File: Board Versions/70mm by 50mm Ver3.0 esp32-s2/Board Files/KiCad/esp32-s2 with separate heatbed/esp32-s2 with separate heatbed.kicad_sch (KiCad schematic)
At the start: 24 parts, among them IC1 ESP32-S2FN4R2, J1 PJ-037B, J2 USB4520-03-0-A, U1 LD1117S33TR_SOT223, U2 MAX31855KASA, Y1 ECS-400-15-33B-CTN-TR

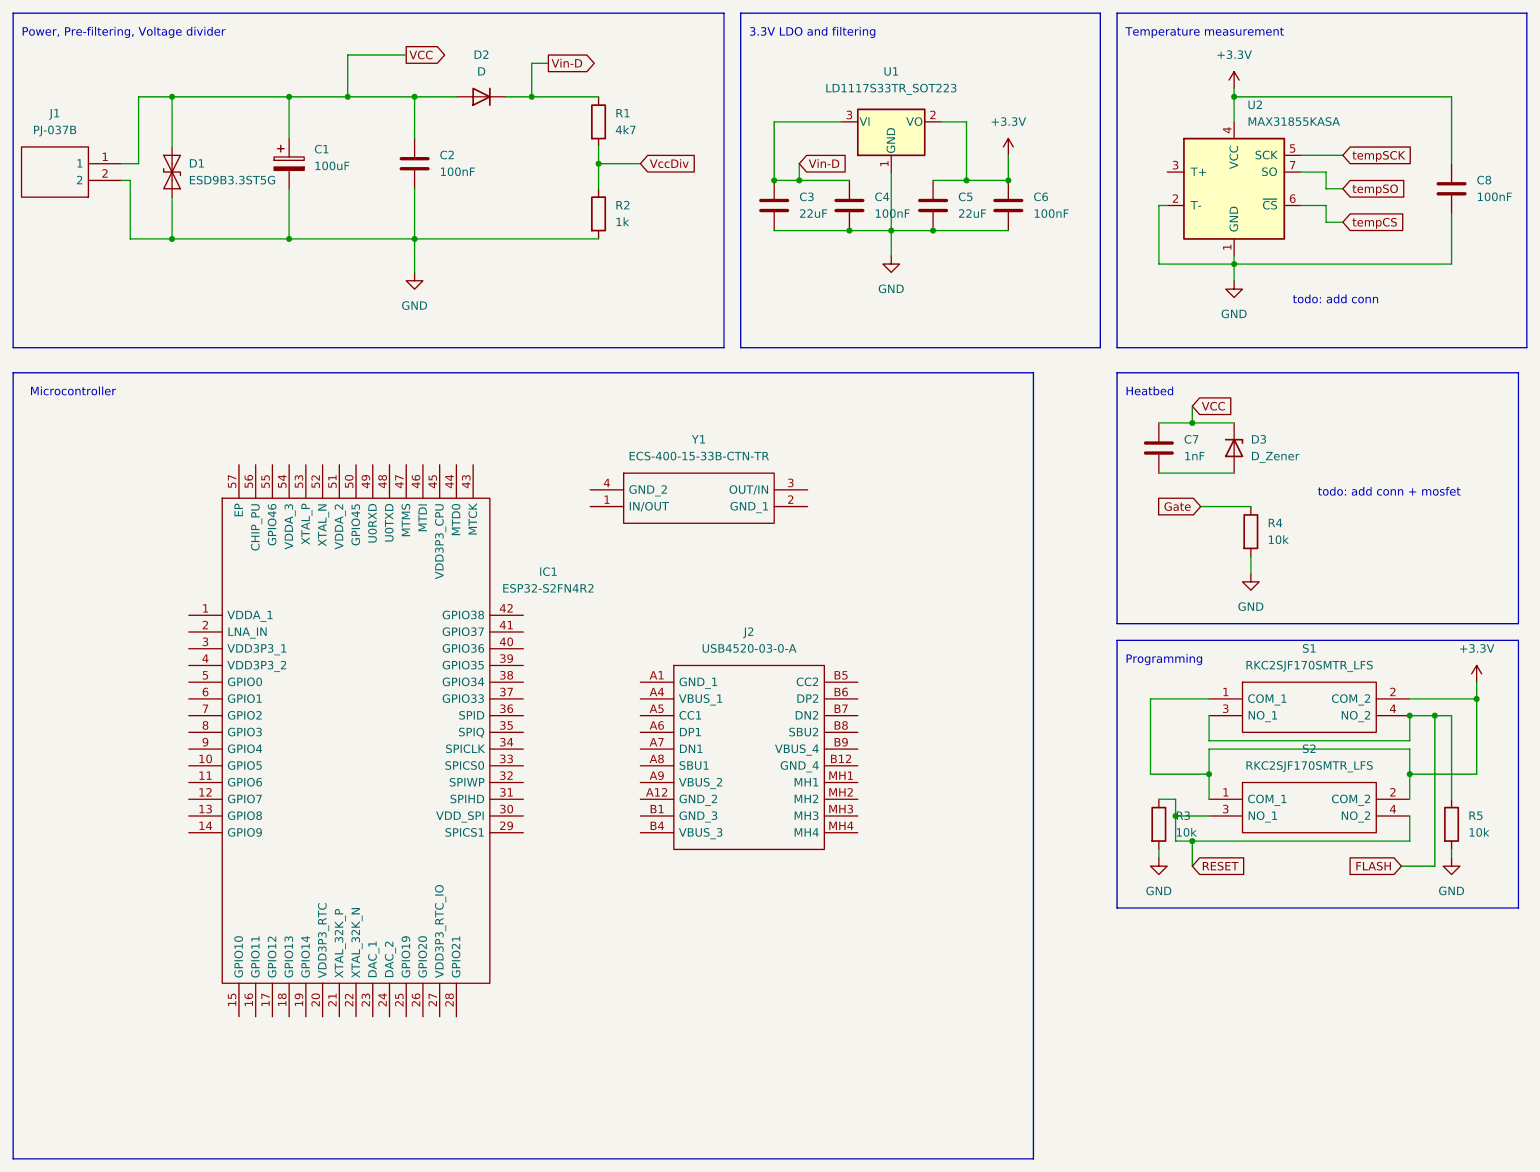
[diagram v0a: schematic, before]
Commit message: Microcontrolling schematics, not complete
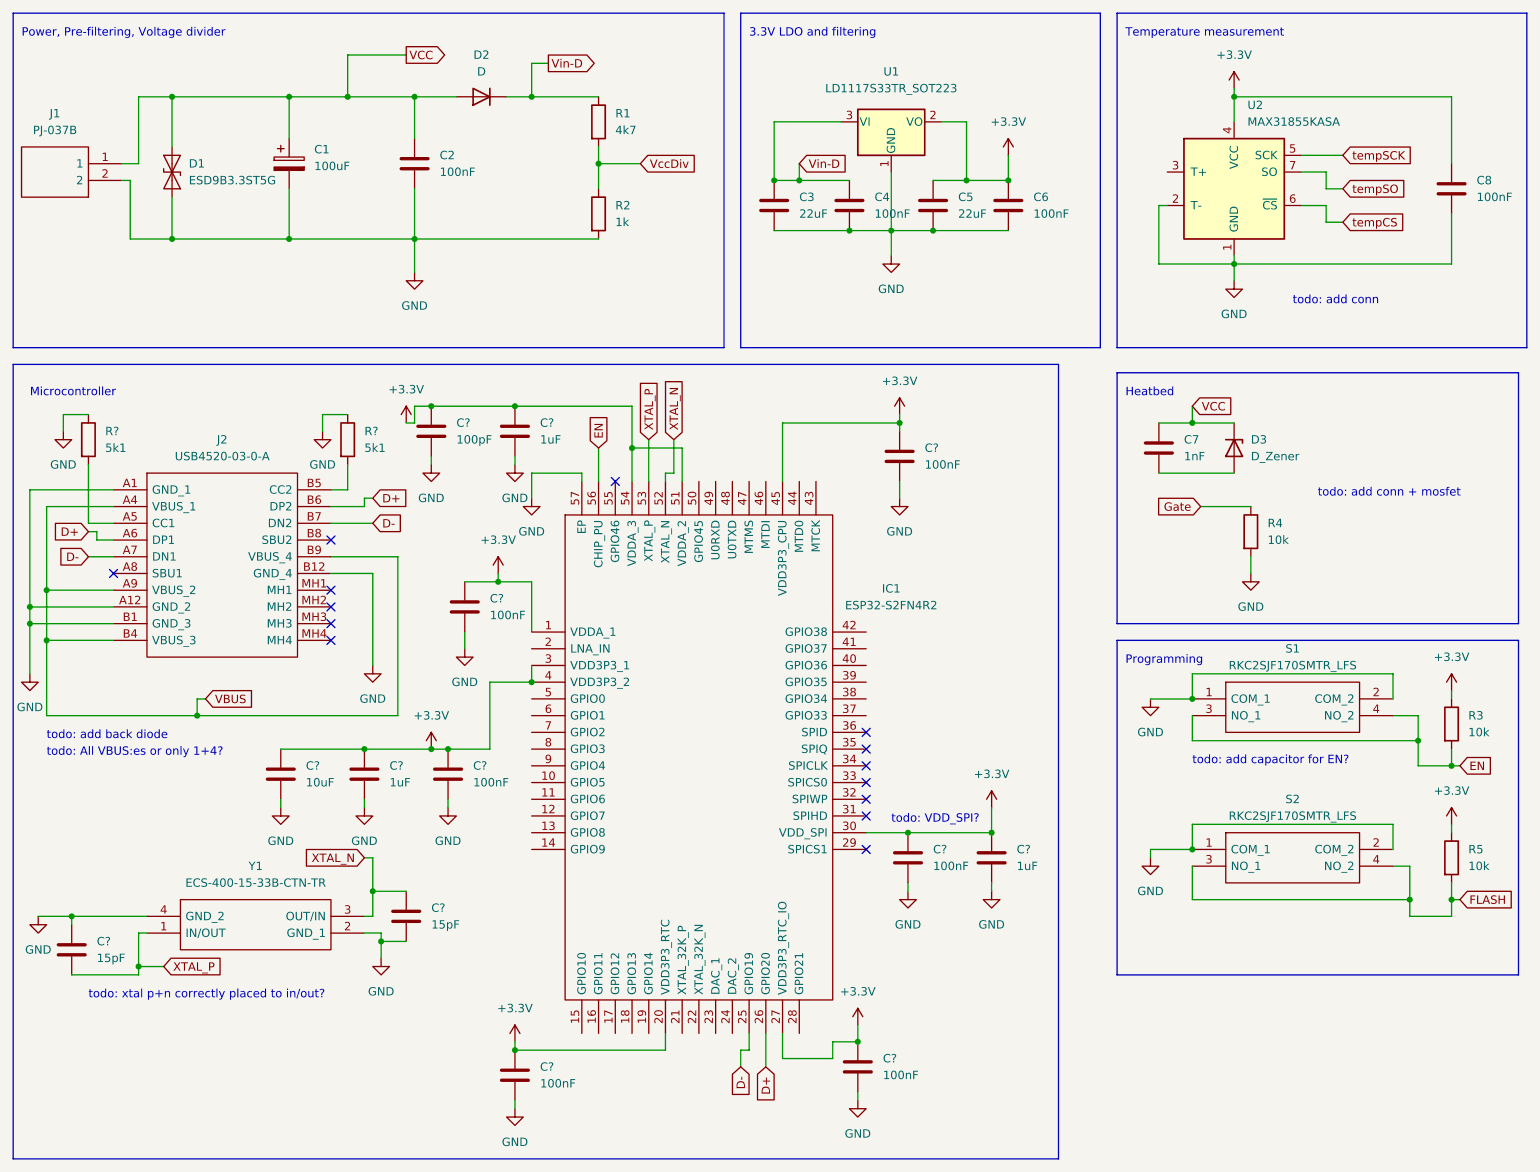
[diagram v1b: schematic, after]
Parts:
- added C? (x6): 100nF, symbol Device:C
- added C?: 10uF, symbol Device:C
- added C? (x2): 15pF, symbol Device:C
- added C?: 100pF, symbol Device:C
- added C? (x3): 1uF, symbol Device:C
- added R? (x2): 5k1, symbol Device:R
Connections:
- net +3V3: now also IC1.1 (VDDA_1), IC1.20 (VDD3P3_RTC), IC1.27 (VDD3P3_RTC_IO), IC1.3 (VDD3P3_1), IC1.30 (VDD_SPI), IC1.4 (VDD3P3_2), IC1.45 (VDD3P3_CPU), IC1.51 (VDDA_2), IC1.54 (VDDA_3), R3.1, R5.1, C?.1, C?.1, C?.1, C?.1, C?.1, C?.1, C?.1, C?.1, C?.1, C?.1, C?.1; no longer S1.1 (COM_1), S1.2 (COM_2), S2.1 (COM_1), S2.2 (COM_2)
- net FLASH: now also R5.2, S2.3 (NO_1), S2.4 (NO_2); no longer R5.1, S1.3 (NO_1), S1.4 (NO_2)
- net GND: now also IC1.57 (EP), J2.A1 (GND_1), J2.A12 (GND_2), J2.B1 (GND_3), J2.B12 (GND_4), S1.1 (COM_1), S1.2 (COM_2), S2.1 (COM_1), S2.2 (COM_2), Y1.2 (GND_1), Y1.4 (GND_2), C?.1, C?.2, C?.2, C?.2, C?.2, C?.2, C?.2, C?.2, C?.2, C?.2, C?.2, C?.2, C?.2, R?.1, R?.1; no longer R3.2, R5.2
- net XTAL_P: now reaches Y1.1 (IN/OUT)
- net XTAL_P: now also IC1.53 (XTAL_P), C?.2
- net XTAL_N: now reaches Y1.3 (OUT/IN)
- net XTAL_N: now also IC1.52 (XTAL_N), C?.1
- net VBUS: now reaches J2.A4 (VBUS_1)
- net VBUS: now also J2.A9 (VBUS_2), J2.B4 (VBUS_3), J2.B9 (VBUS_4)
- net at J2.A5 (CC1): now also R?.2
- net D+: now reaches J2.A6 (DP1)
- net D+: now also IC1.26 (GPIO20), J2.B6 (DP2)
- net D-: now reaches J2.A7 (DN1)
- net D-: now also IC1.25 (GPIO19), J2.B7 (DN2)
- net at J2.B5 (CC2): now also R?.2
- net EN: now reaches IC1.56 (CHIP_PU)
- net EN: now also R3.2, S1.3 (NO_1), S1.4 (NO_2)
- removed net RESET: R3.1, S2.3 (NO_1), S2.4 (NO_2)
- no-connect marks 0 -> 14
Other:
- note added: "todo: All VBUS:es or only 1+4?"
- note added: "todo: VDD_SPI?"
- note added: "todo: add back diode"
- note added: "todo: add capacitor for EN?"
- note added: "todo: xtal p+n correctly placed to in/out?"
- moved on the sheet: IC1, J2, R3, R5, S1, S2, Y1
